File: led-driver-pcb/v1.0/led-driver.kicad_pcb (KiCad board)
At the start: 2 copper layers, 74.4 x 55.8 mm, 37 parts, among them P1 POWER, P2 CTRL, P3 LED, Q1 MOSFET_N, Q2 MOSFET_N, U1 MAX16834

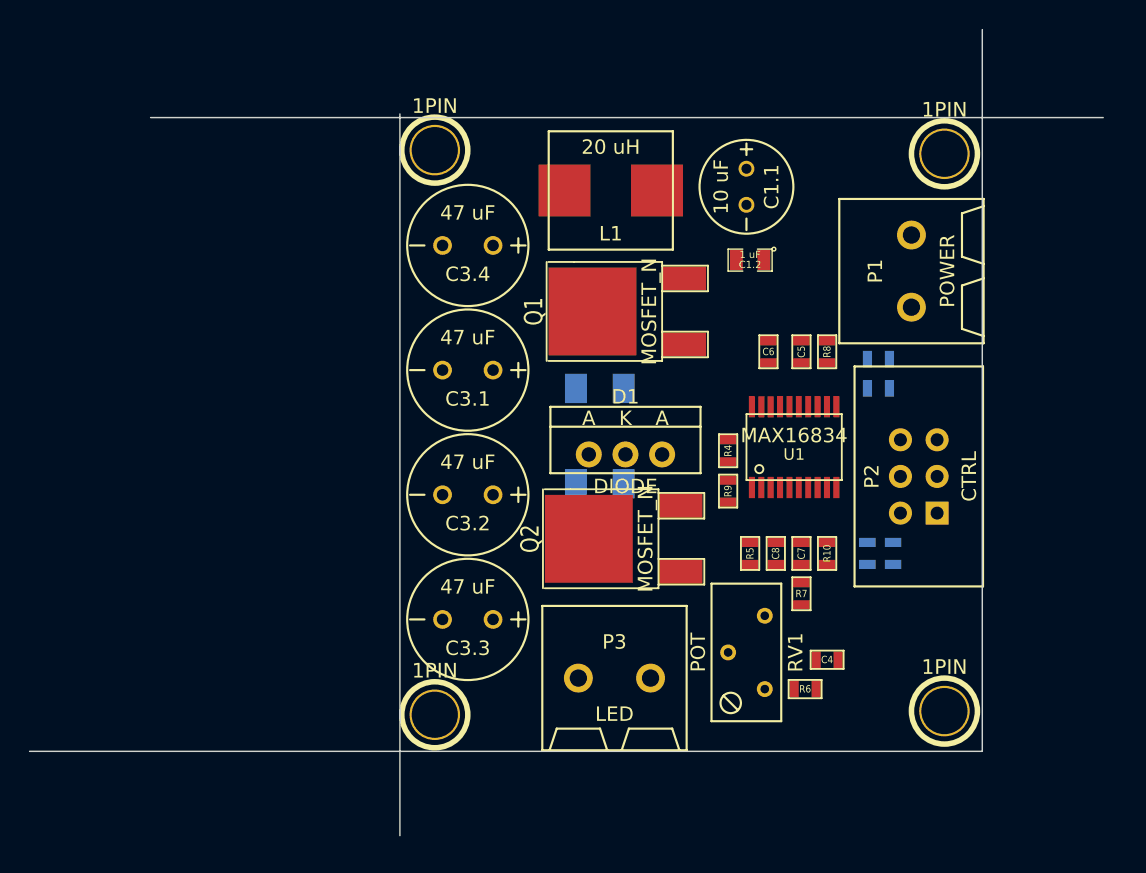
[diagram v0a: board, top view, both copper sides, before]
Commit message: Finished the PCB design.
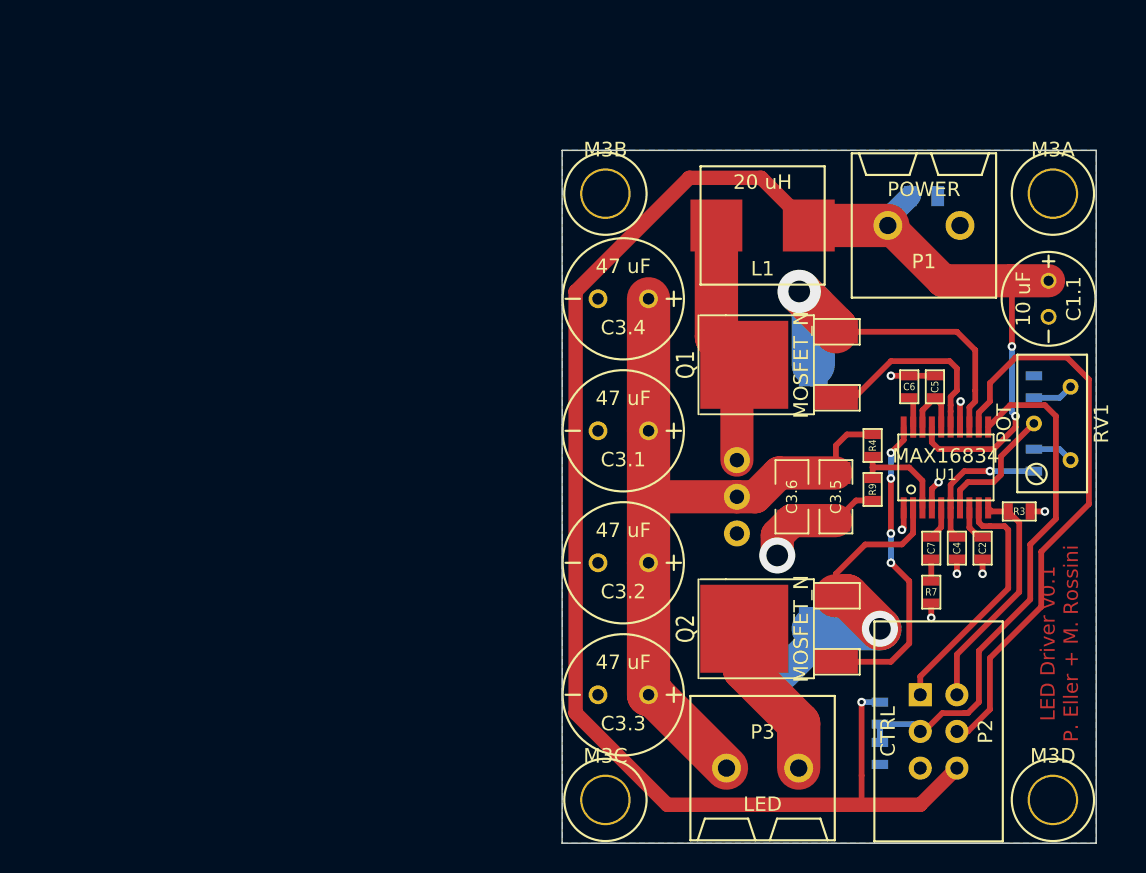
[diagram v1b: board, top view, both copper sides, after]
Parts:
- removed 1PIN (x4): P***, 1pin
- added M3A: P***, 1pin, F.Cu at (213.0, 129.0)
- added M3B: P***, 1pin, F.Cu at (182.0, 129.0)
- added M3C: P***, 1pin, F.Cu at (182.0, 171.0)
- added M3D: P***, 1pin, F.Cu at (213.0, 171.0)
- C1.2, D1, R5, R6: moved to B.Cu
- C2, C3.5, C3.6, R3: moved to F.Cu
- C8: footprint SM0603 -> SM0805; moved to B.Cu
- R10, R8: footprint SM0603 -> SM2512; moved to B.Cu
- moved RV1 26.5 mm to (214.2, 144.9)
- moved R2 25.3 mm to (201.0, 167.8), turned to 270 degrees
- moved R1 24.5 mm to (201.0, 165.0), turned to 270 degrees
- moved R5 22.8 mm to (211.7, 142.4)
- moved R6 22.4 mm to (211.7, 147.5), turned to 90 degrees
- moved C1.1 22.3 mm to (212.7, 136.3)
- moved P2 17.7 mm to (205.1, 166.3), turned to 270 degrees
- moved C3.5 16.4 mm to (198.0, 150.0), turned to 90 degrees
- moved C3.6 15.3 mm to (194.9, 150.0), turned to 90 degrees
- moved C1.2 12.8 mm to (204.1, 129.2)
- moved Q2 12.4 mm to (198.0, 159.1)
- moved P3 12.0 mm to (192.9, 168.8)
- moved C3.3 12.0 mm to (183.2, 163.7)
- moved C4 11.9 mm to (206.3, 153.6), turned to 90 degrees
- moved C3.2 11.8 mm to (183.2, 154.6)
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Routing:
- net N-0000010: track 0.00 -> 181.6 mm, vias 0 -> 3
- net N-0000011: track 0.00 -> 53.4 mm
- net N-000008: track 0.00 -> 40.2 mm
- net N-000005: track 0.00 -> 36.8 mm
- net N-0000022: track 0.00 -> 25.0 mm, vias 0 -> 1
- net N-0000023: track 0.00 -> 22.3 mm, vias 0 -> 1
- net N-0000015: track 0.00 -> 21.5 mm, vias 0 -> 4
- net GND: track 0.00 -> 21.4 mm, vias 0 -> 9
- net N-0000021: track 0.00 -> 17.3 mm
- net N-000004: track 0.00 -> 17.2 mm
- net N-000001: track 0.00 -> 16.3 mm
- net N-0000013: track 0.00 -> 13.9 mm
- net N-0000012: track 0.00 -> 11.2 mm
- net N-000006: track 0.00 -> 9.97 mm, vias 0 -> 1
- net N-000002: track 0.00 -> 9.01 mm
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- added copper zone on B.Cu, net GND
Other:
- board size 74.4 x 55.8 mm -> 37 x 48 mm
- net class Default: clearance 0.254 -> 0.15; trace_width 0.254 -> 0.4; via_dia 0.889 -> 0.6; via_drill 0.635 -> 0.3
- rule trace_clearance: 0.254 -> 0.15
- rule trace_min: 0.254 -> 0.15
- rule via_min_drill: 0.508 -> 0.3
- rule via_min_size: 0.889 -> 0.6
- board text added: "LED Driver v0.1 P. Eller + M. Rossini"
